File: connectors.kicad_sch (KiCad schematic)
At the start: 3 parts, among them J7 Conn_02x25_Counter_Clockwise, J8 Conn_02x25_Counter_Clockwise, J9 35362-0650

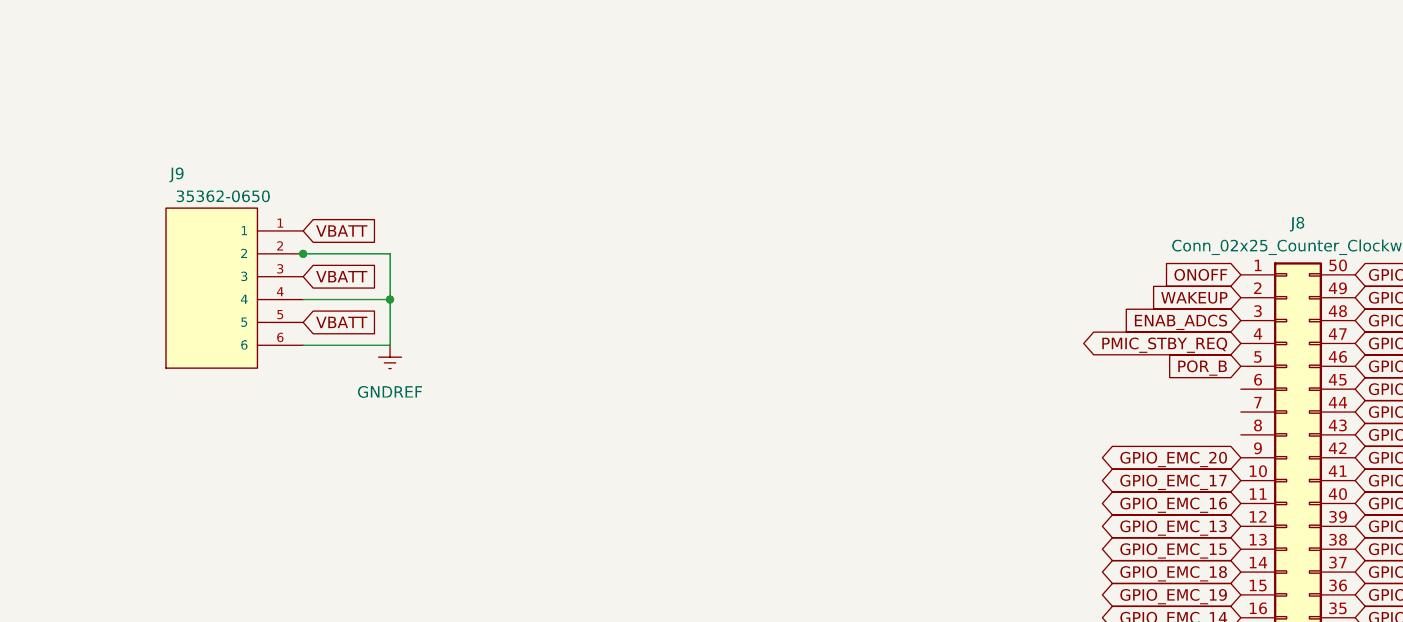
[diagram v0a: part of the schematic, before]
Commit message: hmm
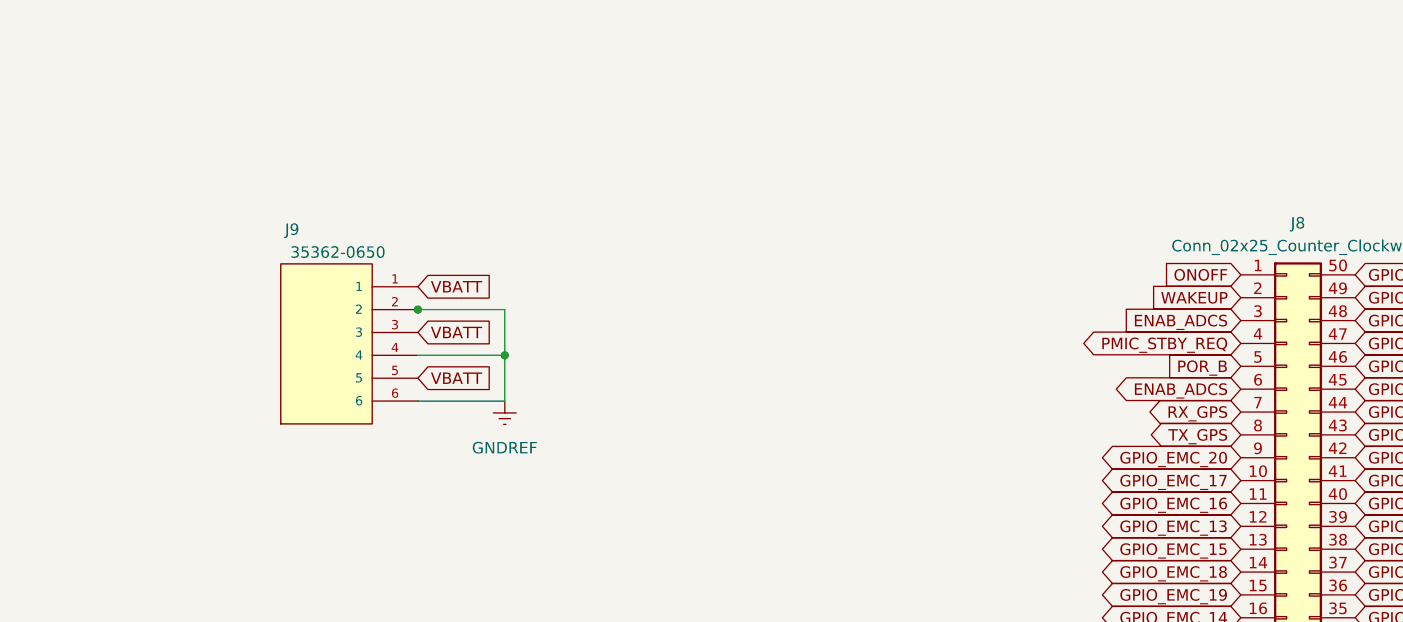
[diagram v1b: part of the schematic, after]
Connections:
- net ENAB_ADCS: now also J8.6 (Pin_6)
- net RX_GPS: now reaches J8.7 (Pin_7)
- net TX_GPS: now reaches J8.8 (Pin_8)
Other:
- moved on the sheet: J9
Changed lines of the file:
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@@
 (kicad_sch (version 20230121) (generator eeschema)
   (paper "USLedger")
-  (junction (at 80.264 109.5248) (diameter 0) (color 0 0 0 0)
-  )
-  (junction (at 70.612 104.4448) (diameter 0) (color 0 0 0 0)
+  (junction (at 93.0148 115.7224) (diameter 0) (color 0 0 0 0)
+  )
+  (junction (at 83.3628 110.6424) (diameter 0) (color 0 0 0 0)
   )
   (bus_entry (at 407.67 18.161) (size -2.54 2.54)
@@
     (stroke (width 0) (type default))
   )
-  (wire (pts (xy 80.264 114.6048) (xy 70.612 114.6048))
-    (stroke (width 0) (type default))
-  )
-  (wire (pts (xy 70.612 104.4448) (xy 80.264 104.4448))
-    (stroke (width 0) (type default))
-  )
-  (wire (pts (xy 80.264 109.5248) (xy 80.264 114.6048))
+  (wire (pts (xy 93.0148 120.8024) (xy 83.3628 120.8024))
+    (stroke (width 0) (type default))
+  )
+  (wire (pts (xy 83.3628 110.6424) (xy 93.0148 110.6424))
+    (stroke (width 0) (type default))
+  )
+  (wire (pts (xy 93.0148 115.7224) (xy 93.0148 120.8024))
     (stroke (width 0) (type default))
   )
@@
     (stroke (width 0) (type default))
   )
-  (wire (pts (xy 80.264 109.5248) (xy 70.612 109.5248))
+  (wire (pts (xy 93.0148 115.7224) (xy 83.3628 115.7224))
     (stroke (width 0) (type default))
   )
@@
     (stroke (width 0) (type default))
   )
-  (wire (pts (xy 70.5612 104.4448) (xy 70.612 104.4448))
+  (wire (pts (xy 83.312 110.6424) (xy 83.3628 110.6424))
     (stroke (width 0) (type default))
   )
@@
     (stroke (width 0) (type default))
   )
-  (wire (pts (xy 80.264 104.4448) (xy 80.264 109.5248))
+  (wire (pts (xy 93.0148 110.6424) (xy 93.0148 115.7224))
     (stroke (width 0) (type default))
   )
@@
     (effects (font (size 1.27 1.27)) (justify left bottom))
   )
-  (global_label "VBATT" (shape input) (at 70.612 106.9848 0) (fields_autoplaced)
-    (effects (font (size 1.27 1.27)) (justify left))
-    (property "Intersheetrefs" "${INTERSHEET_REFS}" (at 78.9796 106.9848 0)
+  (global_label "VBATT" (shape input) (at 83.3628 113.1824 0) (fields_autoplaced)
+    (effects (font (size 1.27 1.27)) (justify left))
+    (property "Intersheetrefs" "${INTERSHEET_REFS}" (at 91.7304 113.1824 0)
       (effects (font (size 1.27 1.27)) (justify left) hide)
     )
@@
     )
   )
+  (global_label "RX_GPS" (shape bidirectional) (at 174.8028 122.0216 180) (fields_autoplaced)
+    (effects (font (size 1.27 1.27)) (justify right))
+    (property "Intersheetrefs" "${INTERSHEET_REFS}" (at 163.5097 122.0216 0)
+      (effects (font (size 1.27 1.27)) (justify right) hide)
+    )
+  )
   (global_label "GPIO_AD_B1_12" (shape bidirectional) (at 187.5028 122.0216 0) (fields_autoplaced)
     (effects (font (size 1.27 1.27)) (justify left))
@@
     )
   )
+  (global_label "ENAB_ADCS" (shape bidirectional) (at 174.8028 119.4816 180) (fields_autoplaced)
+    (effects (font (size 1.27 1.27)) (justify right))
+    (property "Intersheetrefs" "${INTERSHEET_REFS}" (at 160.0625 119.4816 0)
+      (effects (font (size 1.27 1.27)) (justify right) hide)
+    )
+  )
   (global_label "GPIO_EMC_35" (shape bidirectional) (at 187.5028 132.1816 0) (fields_autoplaced)
     (effects (font (size 1.27 1.27)) (justify left))
@@
     )
   )
+  (global_label "TX_GPS" (shape bidirectional) (at 174.8028 124.5616 180) (fields_autoplaced)
+    (effects (font (size 1.27 1.27)) (justify right))
+    (property "Intersheetrefs" "${INTERSHEET_REFS}" (at 163.8121 124.5616 0)
+      (effects (font (size 1.27 1.27)) (justify right) hide)
+    )
+  )
   (global_label "GPIO_B1_05" (shape bidirectional) (at 237.5408 155.448 180) (fields_autoplaced)
     (effects (font (size 1.27 1.27)) (justify right))
@@
     )
   )
-  (global_label "VBATT" (shape input) (at 70.612 112.0648 0) (fields_autoplaced)
-    (effects (font (size 1.27 1.27)) (justify left))
-    (property "Intersheetrefs" "${INTERSHEET_REFS}" (at 78.9796 112.0648 0)
+  (global_label "VBATT" (shape input) (at 83.3628 118.2624 0) (fields_autoplaced)
+    (effects (font (size 1.27 1.27)) (justify left))
+    (property "Intersheetrefs" "${INTERSHEET_REFS}" (at 91.7304 118.2624 0)
       (effects (font (size 1.27 1.27)) (justify left) hide)
     )
@@
     )
   )
-  (global_label "VBATT" (shape input) (at 70.612 101.9048 0) (fields_autoplaced)
-    (effects (font (size 1.27 1.27)) (justify left))
-    (property "Intersheetrefs" "${INTERSHEET_REFS}" (at 78.9796 101.9048 0)
+  (global_label "VBATT" (shape input) (at 83.3628 108.1024 0) (fields_autoplaced)
+    (effects (font (size 1.27 1.27)) (justify left))
+    (property "Intersheetrefs" "${INTERSHEET_REFS}" (at 91.7304 108.1024 0)
       (effects (font (size 1.27 1.27)) (justify left) hide)
     )
@@
     )
   )
-  (symbol (lib_id "mainboard:35362-0650") (at 60.452 109.5248 0) (unit 1)
+  (symbol (lib_id "mainboard:35362-0650") (at 73.2028 115.7224 0) (unit 1)
     (in_bom yes) (on_board yes) (dnp no)
-    (property "Reference" "J9" (at 56.642 95.5548 0)
+    (property "Reference" "J9" (at 69.3928 101.7524 0)
       (effects (font (size 1.27 1.27)))
     )
-    (property "Value" "35362-0650" (at 61.722 98.0948 0)
+    (property "Value" "35362-0650" (at 74.4728 104.2924 0)
       (effects (font (size 1.27 1.27)))
     )
-    (property "Footprint" "mainboard:MOLEX_35362-0650" (at 54.102 118.4148 90)
+    (property "Footprint" "mainboard:MOLEX_35362-0650" (at 66.8528 124.6124 90)
       (effects (font (size 1.27 1.27)) (justify left bottom) hide)
     )
-    (property "Datasheet" "" (at 60.452 109.5248 0)
+    (property "Datasheet" "" (at 73.2028 115.7224 0)
       (effects (font (size 1.27 1.27)) (justify left bottom) hide)
     )
@@
     )
   )
-  (symbol (lib_name "GNDREF_1") (lib_id "power:GNDREF") (at 80.264 114.6556 0) (unit 1)
+  (symbol (lib_name "GNDREF_1") (lib_id "power:GNDREF") (at 93.0148 120.8532 0) (unit 1)
     (in_bom yes) (on_board yes) (dnp no) (fields_autoplaced)
-    (property "Reference" "#PWR033" (at 80.264 121.0056 0)
+    (property "Reference" "#PWR033" (at 93.0148 127.2032 0)
       (effects (font (size 1.27 1.27)) hide)
     )
-    (property "Value" "GNDREF" (at 80.264 119.8372 0)
+    (property "Value" "GNDREF" (at 93.0148 126.0348 0)
       (effects (font (size 1.27 1.27)))
     )
-    (property "Footprint" "" (at 80.264 114.6556 0)
+    (property "Footprint" "" (at 93.0148 120.8532 0)
       (effects (font (size 1.27 1.27)) hide)
     )
-    (property "Datasheet" "" (at 80.264 114.6556 0)
+    (property "Datasheet" "" (at 93.0148 120.8532 0)
       (effects (font (size 1.27 1.27)) hide)
     )
